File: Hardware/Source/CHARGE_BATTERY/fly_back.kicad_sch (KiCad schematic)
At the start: 2 parts, among them U11 AMS1117-5.0, U12 AMS1117-3.3

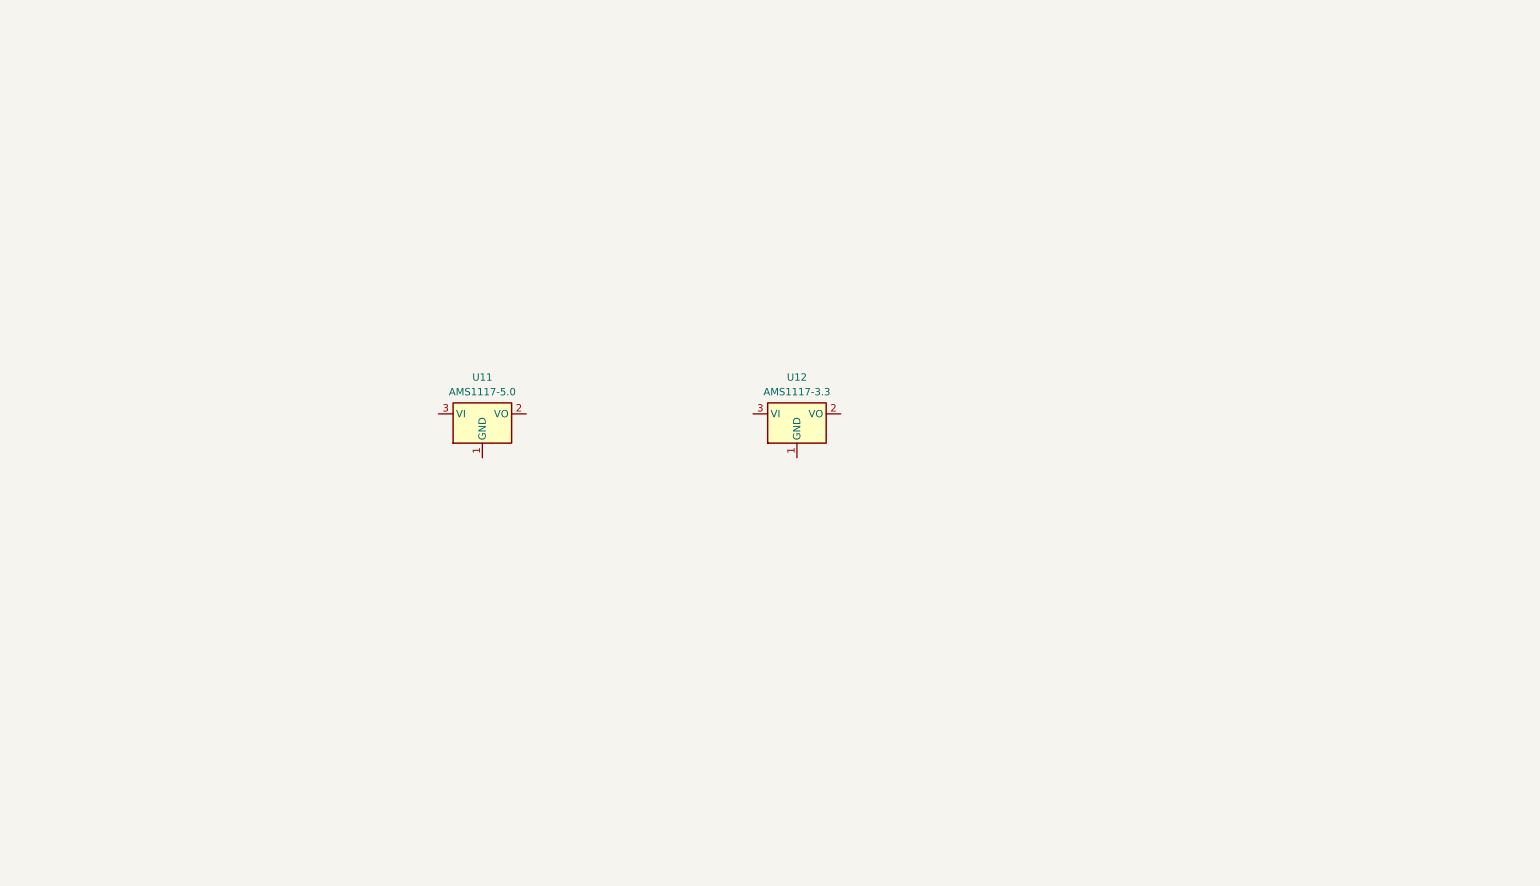
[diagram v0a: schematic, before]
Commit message: Merge branch 'dev_hardware' of https://github.com/DONGKHOA/CHARGE_BATTERY into dev_hardware
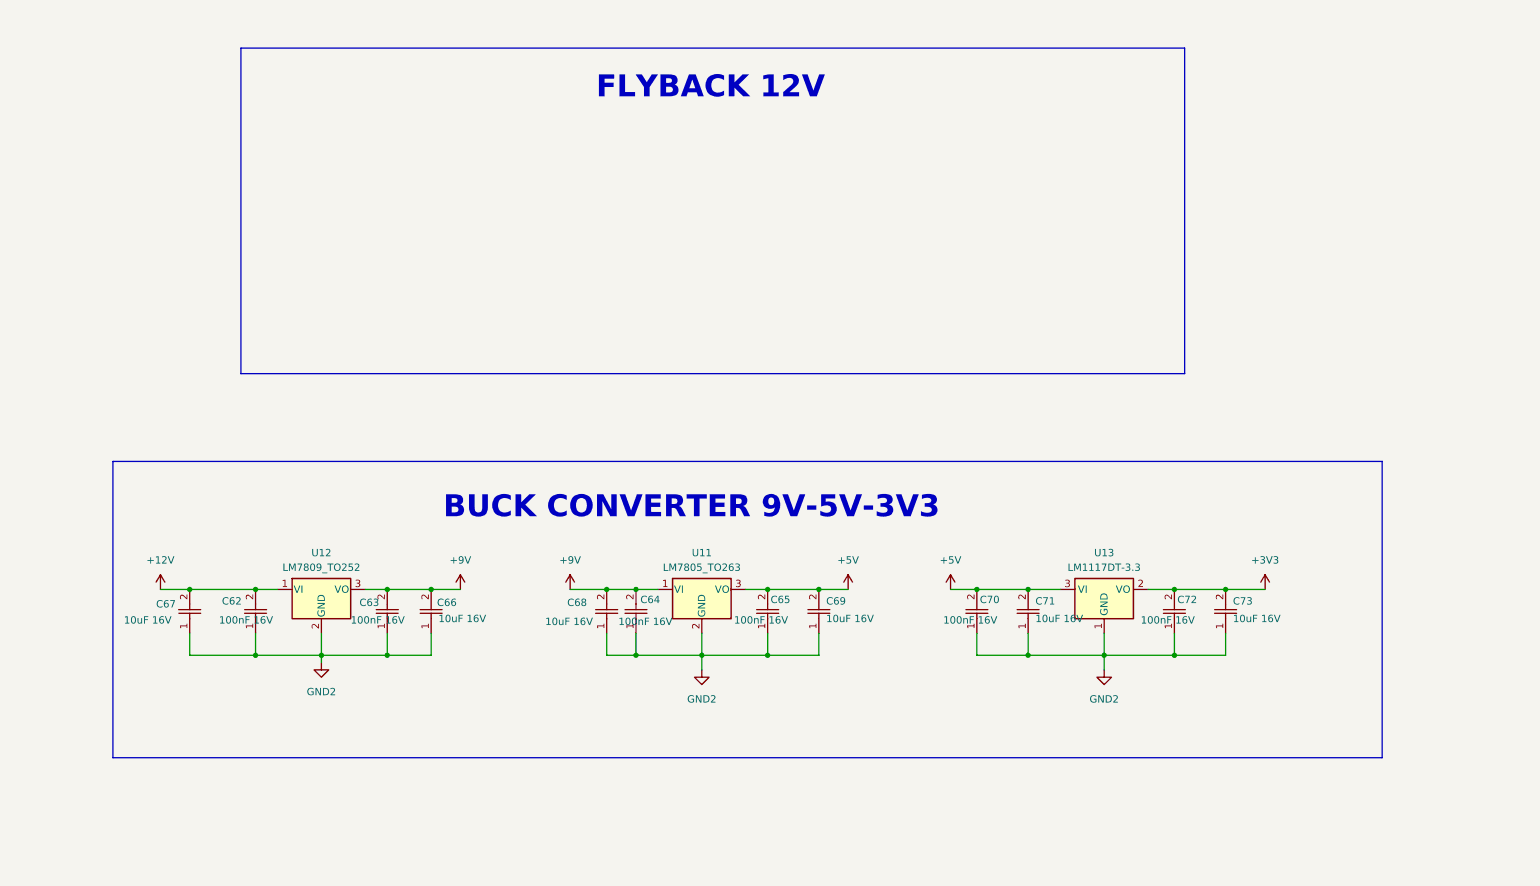
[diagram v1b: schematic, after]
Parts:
- removed U11: AMS1117-5.0, Package_TO_SOT_SMD:SOT-223-3_TabPin2, symbol Regulator_Linear:AMS1117-5.0
- removed U12: AMS1117-3.3, Package_TO_SOT_SMD:SOT-223-3_TabPin2, symbol Regulator_Linear:AMS1117-3.3
- added C62, C63, C64, C65, C70, C72: 100nF 16V, charge_battery_footprint_lib:C_0603_1608Metric, symbol charge_battery_sym_lib:Ceramic_Cap_SMD_100nF_16V
- added C66, C67, C68, C69, C71, C73: 10uF 16V, charge_battery_footprint_lib:Ceramic_Cap_10uF_16V, symbol charge_battery_sym_lib:Ceramic_Cap_SMD_10uF_16V
- added U11: LM7805_TO263, charge_battery_footprint_lib:LM7805_TO-263-3, symbol charge_battery_sym_lib:LM7805_TO263
- added U12: LM7809_TO252, charge_battery_footprint_lib:TO-252-3_TabPin2, symbol charge_battery_sym_lib:LM7809_TO252
- added U13: LM1117DT-3.3, Package_TO_SOT_SMD:TO-252-3_TabPin2, symbol Regulator_Linear:LM1117DT-3.3
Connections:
- new net +12V: C62.2, C67.2, U12.1 (VI)
- new net +3V3: C72.2, C73.2, U13.2 (VO)
- new net +5V: C65.2, C69.2, C70.2, C71.2, U11.3 (VO), U13.3 (VI)
- new net +9V: C63.2, C64.2, C66.2, C68.2, U11.1 (VI), U12.3 (VO)
- new net GND2: C62.1, C63.1, C64.1, C65.1, C66.1, C67.1, C68.1, C69.1, C70.1, C71.1, C72.1, C73.1, U11.2 (GND), U12.2 (GND), U13.1 (GND)
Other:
- note added: "BUCK CONVERTER 9V-5V-3V3"
- note added: "FLYBACK 12V"

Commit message: update flyback lib
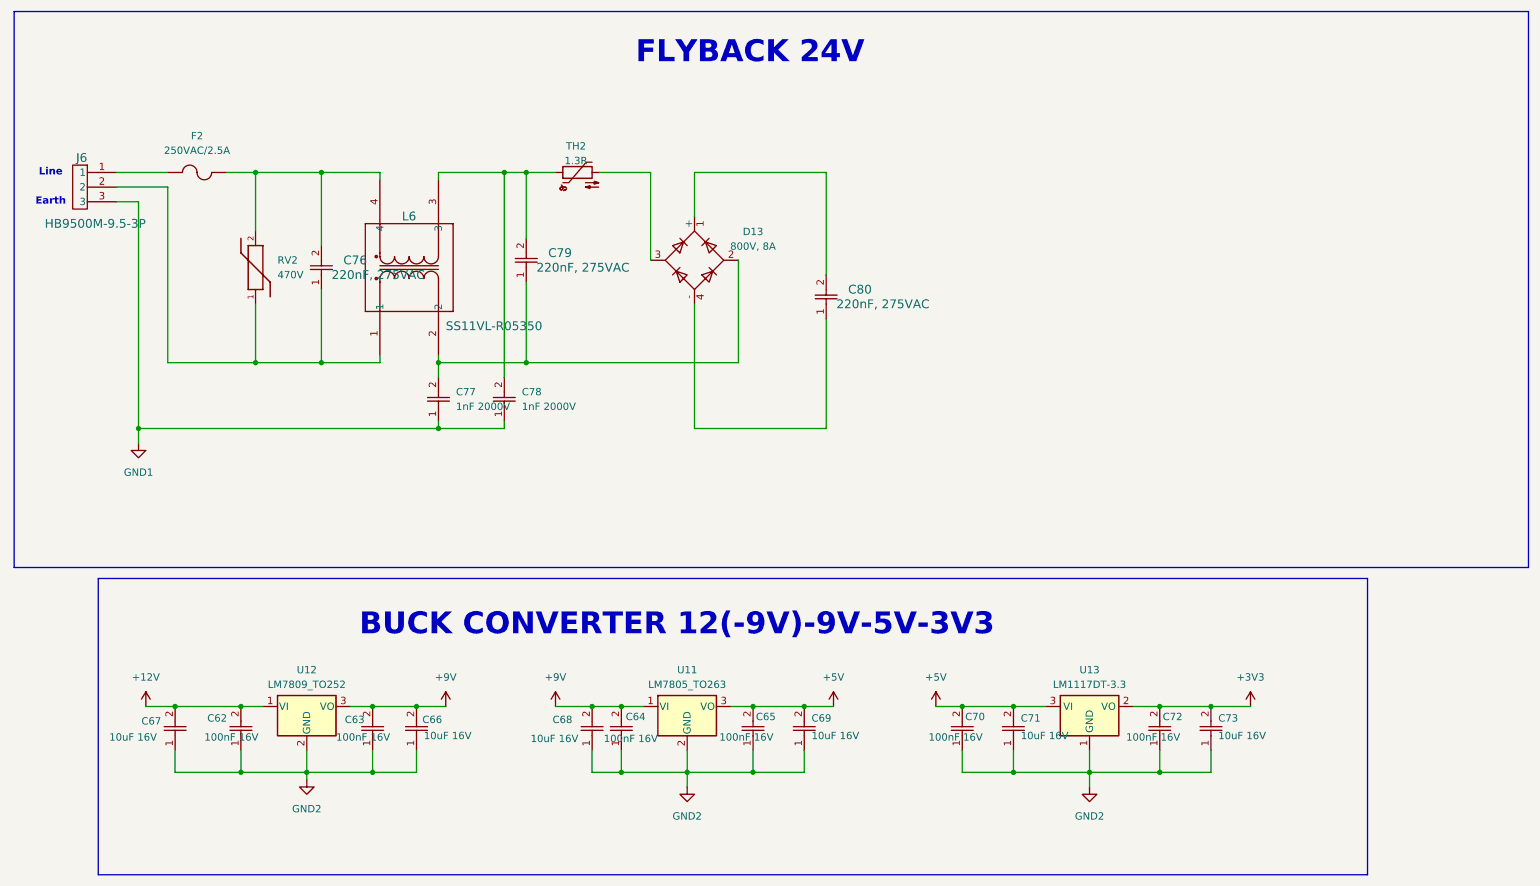
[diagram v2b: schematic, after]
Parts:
- added C76, C79, C80: 220nF, 275VAC, charge_battery_footprint_lib:Candy_Cap_hole_100nF_275V, symbol charge_battery_sym_lib:Film Cap
- added C77, C78: 1nF 2000V, charge_battery_footprint_lib:Ceramic_Cap_Hole_1nF_2000V, symbol charge_battery_sym_lib:Ceramic_Cap_Hole_680pF_1000V
- added D13: 800V, 8A, Diode_THT:Diode_Bridge_Vishay_KBU, symbol charge_battery_sym_lib:KBU808
- added F2: 250VAC/2.5A, charge_battery_footprint_lib:FUSAD2722W65L2250D600, symbol charge_battery_sym_lib:FUSE_250VAC_2.5A
- added J6: HB9500M-9.5-3P, charge_battery_footprint_lib:CONN3_HB9500_KAN, symbol charge_battery_sym_lib:HB9500M-9.5-3P
- added L6: SS11VL-R05350, charge_battery_footprint_lib:IND_SS11VL-R05350_KEM, symbol charge_battery_sym_lib:SS11VL-R05350
- added RV2: 470V, charge_battery_footprint_lib:MOV07D471K, symbol charge_battery_sym_lib:MOV-07D471K
- added TH2: 1.3R, charge_battery_footprint_lib:Thermistor_NTC, symbol charge_battery_sym_lib:Thermistor_NTC
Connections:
- new net: C80.1, D13.4 (-)
- new net: C80.2, D13.1 (+)
- new net: C77.2, C79.1, D13.2, L6.2
- new net: D13.3, TH2.2
- new net: C78.2, C79.2, L6.3, TH2.1
- new net: F2.1, J6.1
- new net: C76.2, F2.2, L6.4, RV2.2
- new net: C76.1, J6.2, L6.1, RV2.1
- new net GND1: C77.1, C78.1, J6.3
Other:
- note added: "BUCK CONVERTER 12(-9V)-9V-5V-3V3"
- note added: "Earth"
- note added: "FLYBACK 24V"
- note added: "Line"
- note removed: "BUCK CONVERTER 9V-5V-3V3"
- note removed: "FLYBACK 12V"
- moved on the sheet: C62, C63, C64, C65, C66, C67, C68, C69, C70, C71, C72, C73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

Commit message: update lib
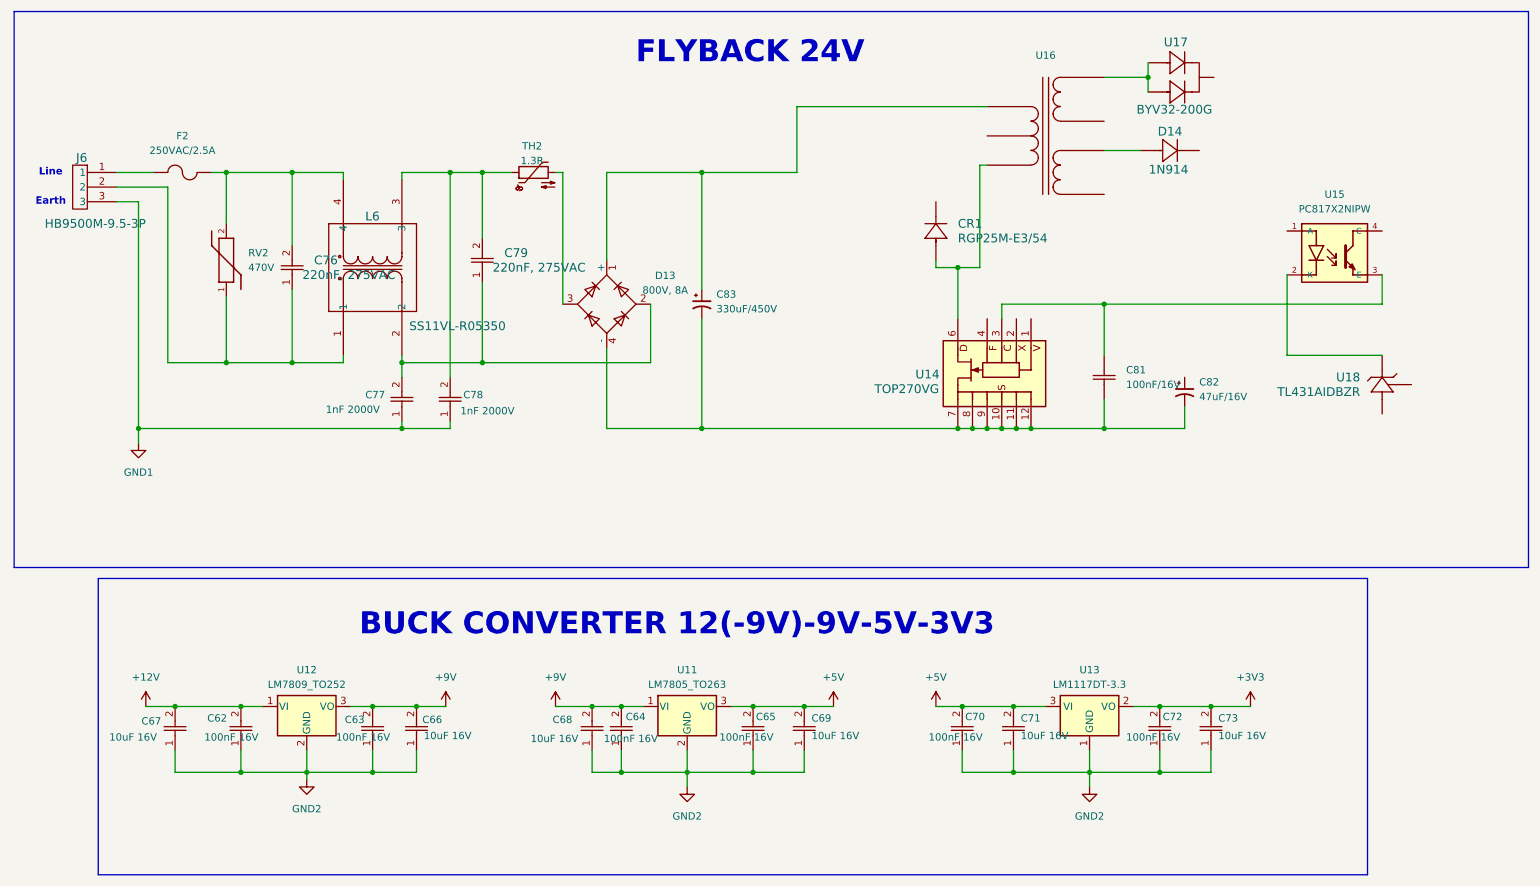
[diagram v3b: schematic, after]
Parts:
- removed C80: 220nF, 275VAC, charge_battery_footprint_lib:Candy_Cap_hole_100nF_275V, symbol charge_battery_sym_lib:Film Cap
- added C81: 100nF/16V, charge_battery_footprint_lib:Ceramic_Cap_0603, symbol charge_battery_sym_lib:Ceramic_Cap_SMD_100nF_16V
- added C82: 47uF/16V, Capacitor_SMD:CP_Elec_5x5.4, symbol charge_battery_sym_lib:Cap_Polarized_SMD_47uF_16V
- added C83: 330uF/450V, charge_battery_footprint_lib:Big_Cap_330uF_450V, symbol charge_battery_sym_lib:Cap_Polarized_330uF_450V
- added CR1: RGP25M-E3/54, charge_battery_footprint_lib:DO-201AD-2, symbol charge_battery_sym_lib:RGP25M-E3_54
- added D14: 1N914, AFL-W2C8.9D, symbol charge_battery_sym_lib:1N914
- added U14: TOP270VG, charge_battery_footprint_lib:eDIP-12B_PWI, symbol charge_battery_sym_lib:TOP270VG
- added U15: PC817X2NIPW, charge_battery_footprint_lib:PC817X2NIPW, symbol charge_battery_sym_lib:PC817X2NIPW
- added U16: ~, symbol charge_battery_sym_lib:Transformer_flyback
- added U17: BYV32-200G, charge_battery_footprint_lib:TO-220-3, symbol charge_battery_sym_lib:BYV32-200G
- added U18: TL431AIDBZR, charge_battery_footprint_lib:SOT23, symbol charge_battery_sym_lib:TL431AIDBZR
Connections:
- net at D13.4 (-): now also C81.1, C82.2, C83.2, U14.10 (S), U14.11 (S), U14.12 (S), U14.7 (S), U14.8 (S), U14.9 (S)
- net at D13.1 (+): now also C83.1, U16.1 (IN+)
- new net: U15.2 (K), U18.1 (K)
- new net: U16.4 (OUT1A), U17.1 (A), U17.3 (A)
- new net: C81.2, U14.3 (C), U15.3 (E)
- new net: CR1.2 (A), U14.6 (D), U16.3 (IN-)
- new net: D14., U16.6 (OUT2A)
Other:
- moved on the sheet: C76, C77, C78, C79, D13, F2, L6, RV2, TH2
